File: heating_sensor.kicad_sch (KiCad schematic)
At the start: 3 parts

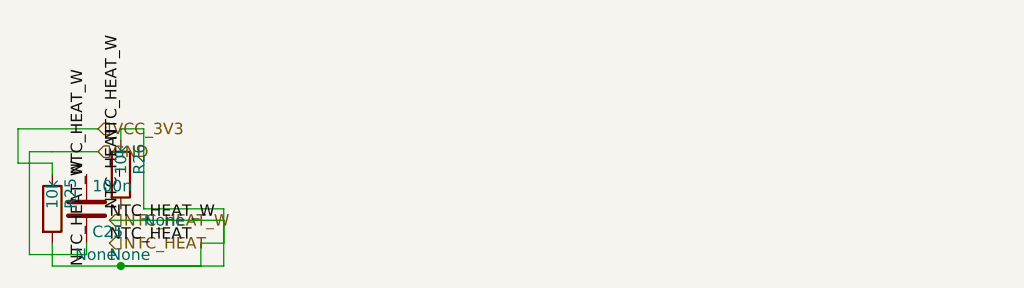
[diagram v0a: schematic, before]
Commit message: tests_fix
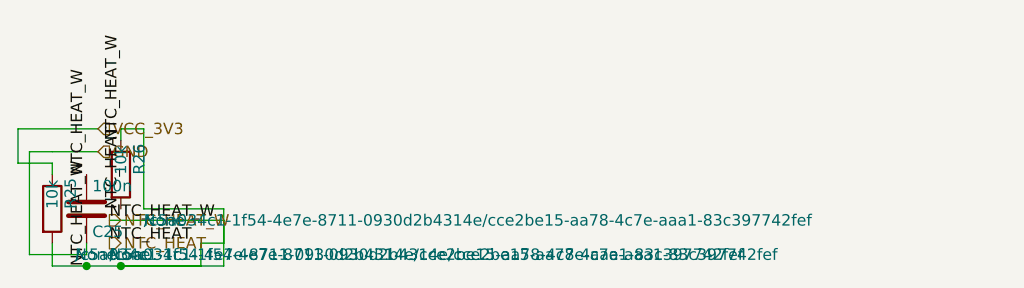
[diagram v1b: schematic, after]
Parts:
- C25, R25, R26: hierarchy_path (none) -> /c5a034c1-1f54-4e7e-8711-0930d2b4314e/cce2be15-aa78-4c7e-aa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
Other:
- title: (none) -> climate_control_niva_travel
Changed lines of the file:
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@@
 	(generator_version "9.0")
 	(paper "A4")
+	(title_block
+		(title "climate_control_niva_travel")
+	)
 	(symbol
 		(lib_id "Device:C")
@@
 			)
 		)
+		(property "hierarchy_path" "/c5a034c1-1f54-4e7e-8711-0930d2b4314e/cce2be15-aa78-4c7e-aaa1-83c397742fef"
+			(at 20.32 22.8599 0)
+			(effects
+				(font
+					(size 1.27 1.27)
+				)
+				(justify left)
+			)
+		)
 		(pin "1"
 		)
@@
 		)
 		(instances
-			(project "Untitled"
-				(path "/7edcb6ac-6215-4f27-8410-70bd096f4d3f"
+			(project "climate_control_niva_travel"
+				(path "/c5a034c1-1f54-4e7e-8711-0930d2b4314e/cce2be15-aa78-4c7e-aaa1-83c397742fef"
 					(reference "C25")
 					(unit 1)
@@
 			)
 		)
+		(property "hierarchy_path" "/c5a034c1-1f54-4e7e-8711-0930d2b4314e/cce2be15-aa78-4c7e-aaa1-83c397742fef"
+			(at 16.51 22.8599 0)
+			(effects
+				(font
+					(size 1.27 1.27)
+				)
+				(justify left)
+			)
+		)
 		(pin "1"
 		)
@@
 		)
 		(instances
-			(project "Untitled"
-				(path "/7edcb6ac-6215-4f27-8410-70bd096f4d3f"
-					(reference "R25")
+			(project "climate_control_niva_travel"
+				(path "/c5a034c1-1f54-4e7e-8711-0930d2b4314e/cce2be15-aa78-4c7e-aaa1-83c397742fef"
+					(reference "R41")
 					(unit 1)
 				)
@@
 			)
 		)
+		(property "hierarchy_path" "/c5a034c1-1f54-4e7e-8711-0930d2b4314e/cce2be15-aa78-4c7e-aaa1-83c397742fef"
+			(at 24.13 19.0499 0)
+			(effects
+				(font
+					(size 1.27 1.27)
+				)
+				(justify left)
+			)
+		)
 		(pin "1"
 		)
@@
 		)
 		(instances
-			(project "Untitled"
-				(path "/7edcb6ac-6215-4f27-8410-70bd096f4d3f"
-					(reference "R26")
+			(project "climate_control_niva_travel"
+				(path "/c5a034c1-1f54-4e7e-8711-0930d2b4314e/cce2be15-aa78-4c7e-aaa1-83c397742fef"
+					(reference "R42")
 					(unit 1)
 				)
@@
 			(type default)
 		)
+	)
+	(junction
+		(at 17.78 24.13)
+		(diameter 0)
+		(color 0 0 0 0)
 	)
 	(junction
@@
 	)
 	(hierarchical_label "NTC_HEAT_W"
-		(shape input)
+		(shape output)
 		(at 20.32 19.05 0)
 		(effects
@@
 	)
 	(hierarchical_label "NTC_HEAT"
-		(shape input)
+		(shape output)
 		(at 20.32 21.59 0)
 		(effects

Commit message: refactoring
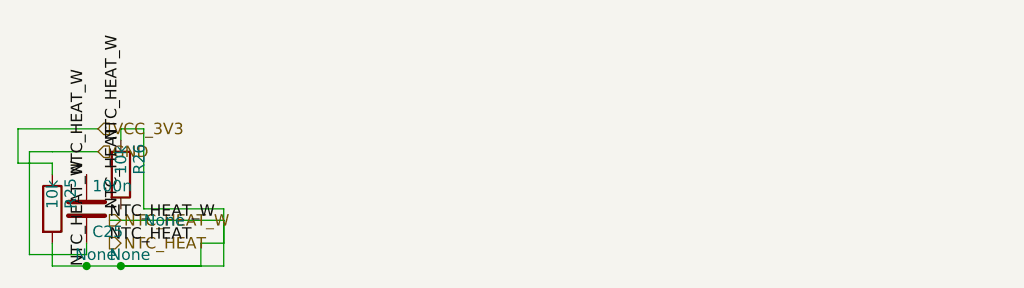
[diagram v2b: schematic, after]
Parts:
- C25, R25, R26: hierarchy_path /c5a034c1-1f54-4e7e-8711-0930d2b4314e/cce2be15-aa78-4c7e-aa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 -> (none)
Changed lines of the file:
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@@
-			)
-		)
-		(property "hierarchy_path" "/c5a034c1-1f54-4e7e-8711-0930d2b4314e/cce2be15-aa78-4c7e-aaa1-83c397742fef"
-			(at 20.32 22.8599 0)
-			(effects
-				(font
-					(size 1.27 1.27)
-				)
-				(justify left)
 			)
 		)
@@
 		(instances
 			(project "climate_control_niva_travel"
-				(path "/c5a034c1-1f54-4e7e-8711-0930d2b4314e/cce2be15-aa78-4c7e-aaa1-83c397742fef"
-					(reference "C25")
+				(path "/165a98f1-2dde-4141-9fdc-c935d39c8cff/2827009f-f2b8-443b-9f5b-0ad26ce039e9/"
+					(reference "C0425")
 					(unit 1)
 				)
@@
 			)
 		)
-		(property "hierarchy_path" "/c5a034c1-1f54-4e7e-8711-0930d2b4314e/cce2be15-aa78-4c7e-aaa1-83c397742fef"
-			(at 16.51 22.8599 0)
-			(effects
-				(font
-					(size 1.27 1.27)
-				)
-				(justify left)
-			)
-		)
 		(pin "1"
 		)
@@
 		(instances
 			(project "climate_control_niva_travel"
-				(path "/c5a034c1-1f54-4e7e-8711-0930d2b4314e/cce2be15-aa78-4c7e-aaa1-83c397742fef"
-					(reference "R41")
+				(path "/165a98f1-2dde-4141-9fdc-c935d39c8cff/2827009f-f2b8-443b-9f5b-0ad26ce039e9/"
+					(reference "R0425")
 					(unit 1)
 				)
@@
 			)
 		)
-		(property "hierarchy_path" "/c5a034c1-1f54-4e7e-8711-0930d2b4314e/cce2be15-aa78-4c7e-aaa1-83c397742fef"
-			(at 24.13 19.0499 0)
-			(effects
-				(font
-					(size 1.27 1.27)
-				)
-				(justify left)
-			)
-		)
 		(pin "1"
 		)
@@
 		(instances
 			(project "climate_control_niva_travel"
-				(path "/c5a034c1-1f54-4e7e-8711-0930d2b4314e/cce2be15-aa78-4c7e-aaa1-83c397742fef"
-					(reference "R42")
+				(path "/165a98f1-2dde-4141-9fdc-c935d39c8cff/2827009f-f2b8-443b-9f5b-0ad26ce039e9/"
+					(reference "R0426")
 					(unit 1)
 				)

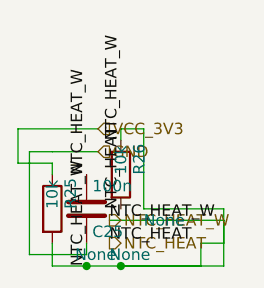
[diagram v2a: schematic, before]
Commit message: refactoring
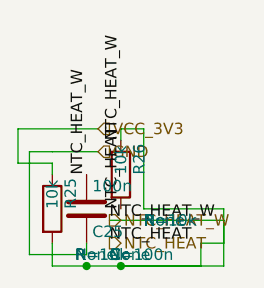
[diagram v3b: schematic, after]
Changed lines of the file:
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@@
+			)
+		)
+		(property "Sim.Device" "C"
+			(at 20.32 22.8599 0)
+			(effects
+				(font
+					(size 1.27 1.27)
+				)
+				(justify left)
+			)
+		)
+		(property "Sim.Params" "C=100n"
+			(at 20.32 22.8599 0)
+			(effects
+				(font
+					(size 1.27 1.27)
+				)
+				(justify left)
 			)
 		)
@@
 		(instances
 			(project "climate_control_niva_travel"
-				(path "/165a98f1-2dde-4141-9fdc-c935d39c8cff/2827009f-f2b8-443b-9f5b-0ad26ce039e9/"
+				(path "/cc416b40-1361-4232-ac1e-5cd36ef0c0fb/4058bf07-d3ed-47ea-a155-e5643b2095d0/"
 					(reference "C0425")
 					(unit 1)
@@
 			)
 		)
+		(property "Sim.Device" "R"
+			(at 16.51 22.8599 0)
+			(effects
+				(font
+					(size 1.27 1.27)
+				)
+				(justify left)
+			)
+		)
+		(property "Sim.Params" "R=10k"
+			(at 16.51 22.8599 0)
+			(effects
+				(font
+					(size 1.27 1.27)
+				)
+				(justify left)
+			)
+		)
 		(pin "1"
 		)
@@
 		(instances
 			(project "climate_control_niva_travel"
-				(path "/165a98f1-2dde-4141-9fdc-c935d39c8cff/2827009f-f2b8-443b-9f5b-0ad26ce039e9/"
+				(path "/cc416b40-1361-4232-ac1e-5cd36ef0c0fb/4058bf07-d3ed-47ea-a155-e5643b2095d0/"
 					(reference "R0425")
 					(unit 1)
@@
 			)
 		)
+		(property "Sim.Device" "R"
+			(at 24.13 19.0499 0)
+			(effects
+				(font
+					(size 1.27 1.27)
+				)
+				(justify left)
+			)
+		)
+		(property "Sim.Params" "R=10k"
+			(at 24.13 19.0499 0)
+			(effects
+				(font
+					(size 1.27 1.27)
+				)
+				(justify left)
+			)
+		)
 		(pin "1"
 		)
@@
 		(instances
 			(project "climate_control_niva_travel"
-				(path "/165a98f1-2dde-4141-9fdc-c935d39c8cff/2827009f-f2b8-443b-9f5b-0ad26ce039e9/"
+				(path "/cc416b40-1361-4232-ac1e-5cd36ef0c0fb/4058bf07-d3ed-47ea-a155-e5643b2095d0/"
 					(reference "R0426")
 					(unit 1)
@@
 	(junction
 		(at 17.78 24.13)
-		(diameter 0)
+		(diameter 0.0000)
 		(color 0 0 0 0)
 	)
 	(junction
 		(at 21.59 24.13)
-		(diameter 0)
+		(diameter 0.0000)
 		(color 0 0 0 0)
 	)
@@
 		(effects
 			(font
-				(size 1.27 1.27)
-			)
-			(justify left bottom)
-		)
-	)
-	(label "NTC_HEAT_W"
-		(at 17.78 24.13 90)
-		(effects
-			(font
